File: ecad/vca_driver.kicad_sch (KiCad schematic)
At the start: 18 parts, among them Q2 BD140, Q4 BD139, U3 OPA2277

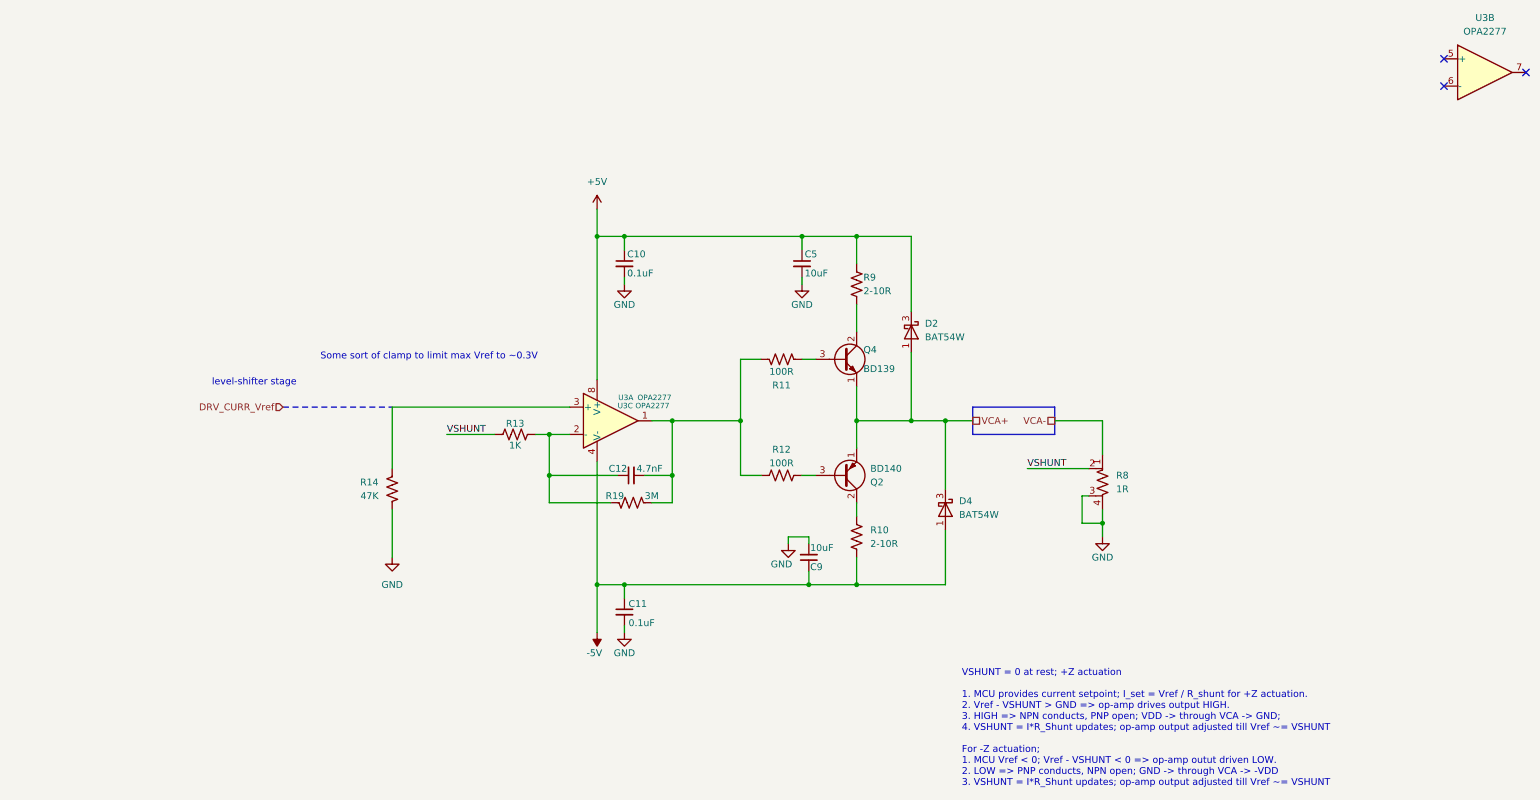
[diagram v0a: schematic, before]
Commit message: vca drivec almost done
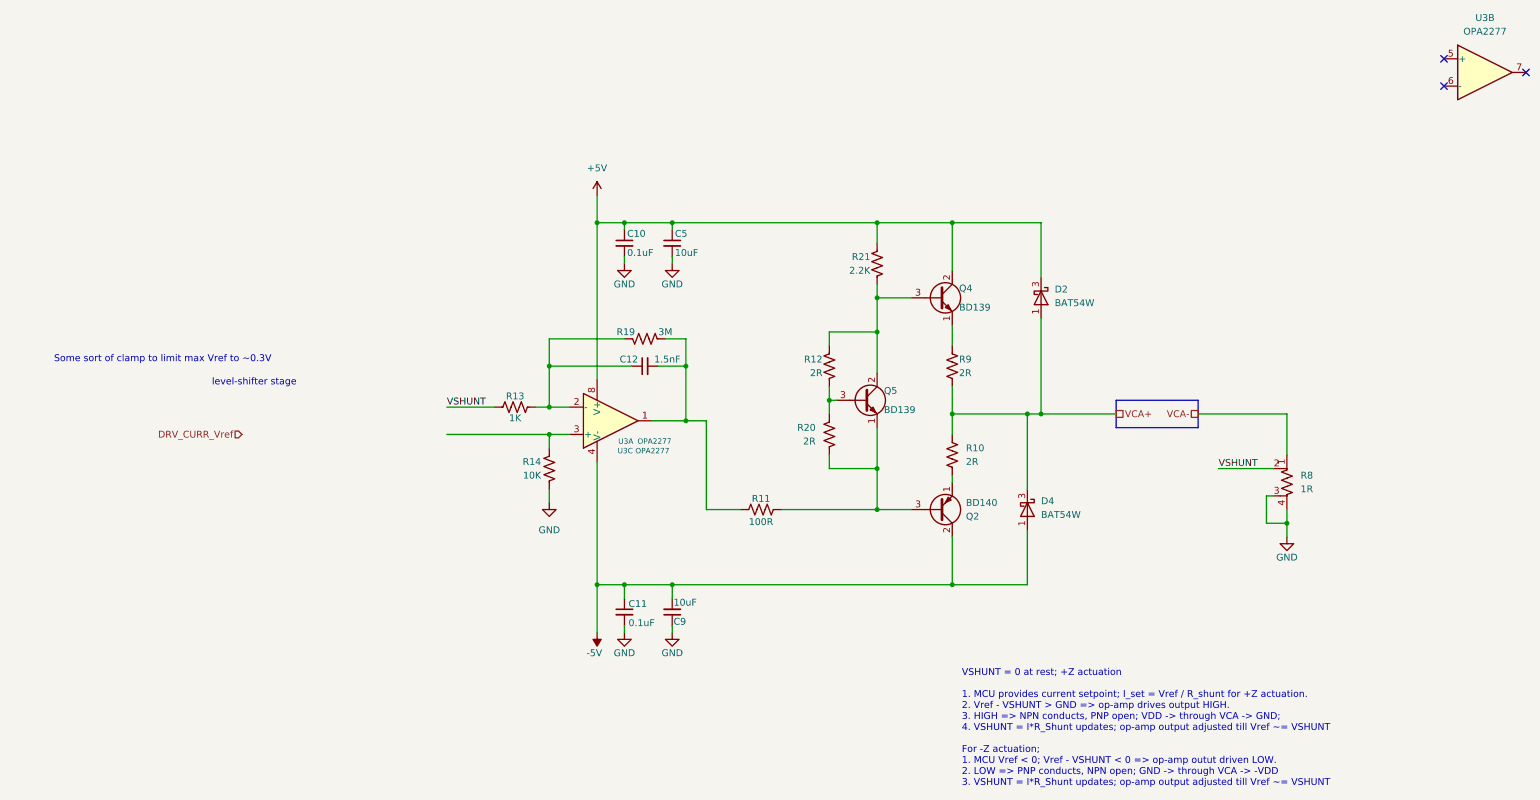
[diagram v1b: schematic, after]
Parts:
- added Q5: BD139, Package_TO_SOT_THT:TO-126-3_Vertical, symbol Transistor_BJT:BD139
- added R20: 2R, symbol Device:R_US
- added R21: 2.2K, symbol Device:R_US
- C12: value 4.7nF -> 1.5nF
- R10, R9: value 2-10R -> 2R
- R12: value 100R -> 2R
- R14: value 47K -> 10K
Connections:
- net +5V: now also Q4.2 (C), R21.1; no longer R9.1
- net -5V: now also C9.2, Q2.2 (C); no longer C9.1, R10.2
- net GND: now also C9.1; no longer C9.2
- net VCA+: now also R10.1, R9.2; no longer Q2.1 (E), Q4.1 (E)
- net at C12.2, R11.2, R19.2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: no longer R12.2
- net at R12.1: now also Q4.3 (B), Q5.2 (C), R21.2; no longer Q2.3 (B)
- net at R11.1: now also Q2.3 (B), Q5.1 (E), R20.2; no longer Q4.3 (B)
- new net: Q5.3 (B), R12.2, R20.1
- new net: Q4.1 (E), R9.1
- new net: Q2.1 (E), R10.2
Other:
- moved on the sheet: C10, C12, C5, C9, D2, D4, Q2, Q4, R10, R11, R13, R14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
